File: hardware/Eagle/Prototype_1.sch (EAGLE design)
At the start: 11 parts, among them IC1 MEGA32-P, Q1 16MHz

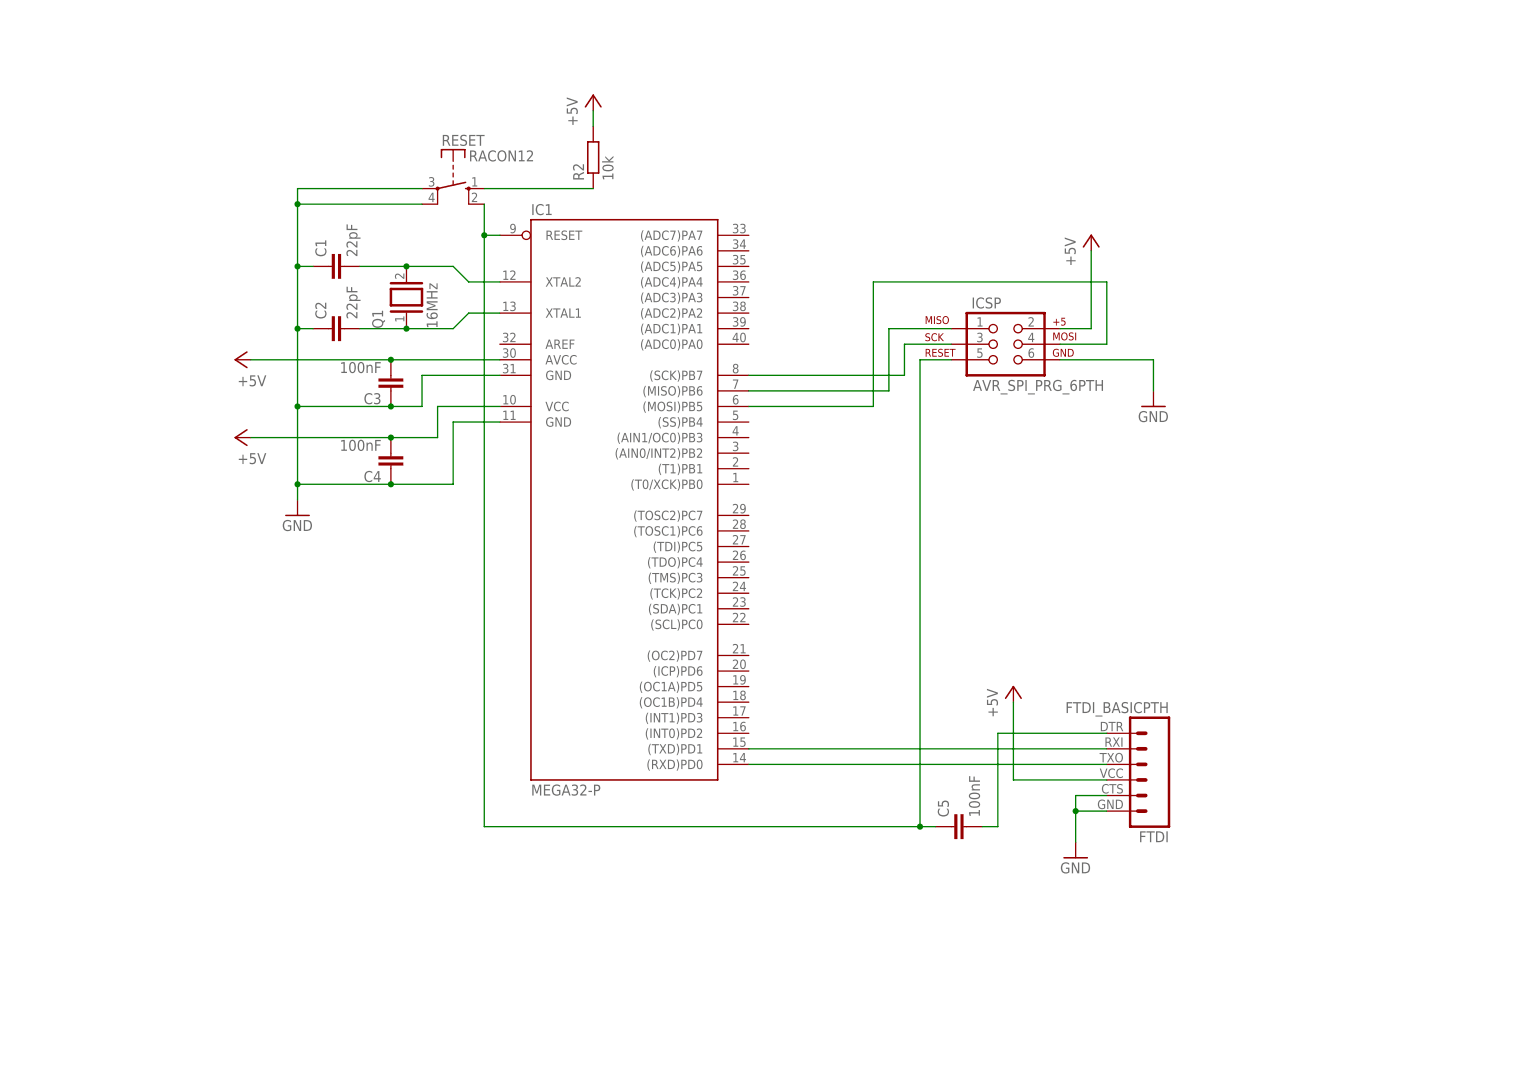
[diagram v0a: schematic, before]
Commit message: Readme and Eagle Circuit Files updated
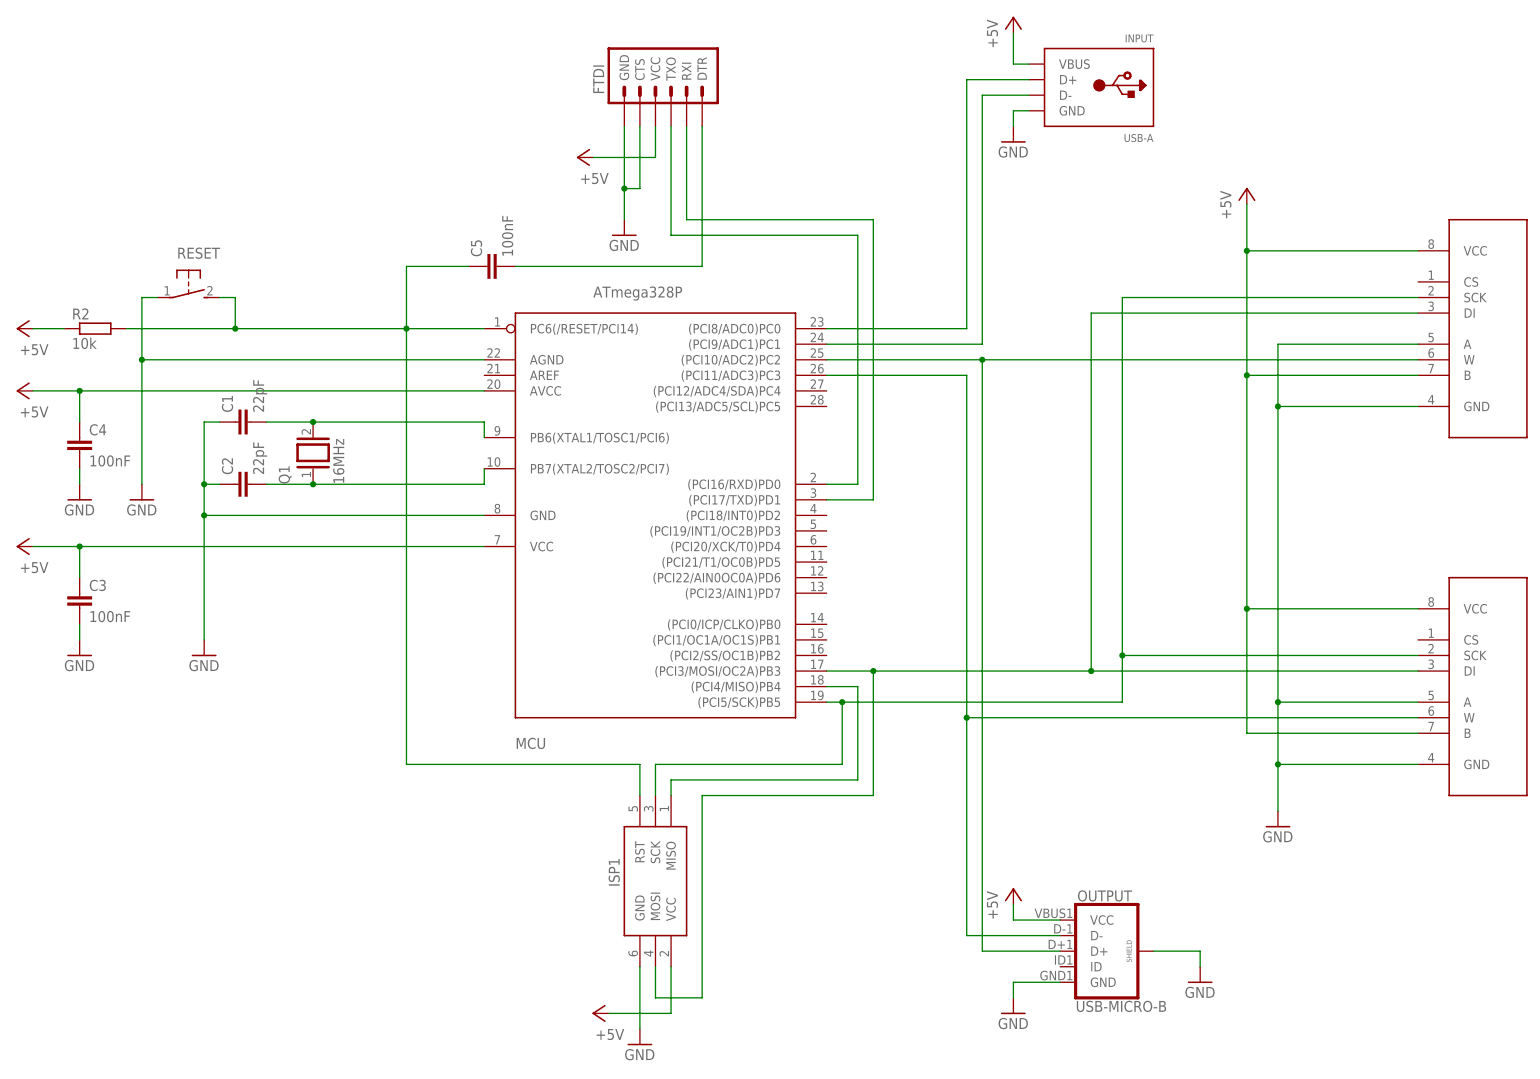
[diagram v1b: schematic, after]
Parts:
- removed IC1: MEGA32-P, atmel:MEGA32-P
- removed ICSP: AVR_SPI_PRG_6PTH, SparkFun-Connectors:AVR_SPI_PRG_6PTH
- added INPUT: USB-A, adafruit:USB-A
- added ISP1: AVRISP-6, adafruit:AVRISP-6
- added MCU: ATmega328P, adafruit:ATMEGA168-20P
- added OUTPUT: USB-MICRO-B, SparkFun-Connectors:USB_MICROB_PLUGCONN-11752
- added POTI, POTI1: MCP41XXXDIL, SparkFun-AnalogIC:MCP41XXXDIL
- FTDI: value FTDI_BASICPTH -> (none); device SparkFun-Connectors:FTDI_BASICPTH -> SparkFun-Connectors:ARDUINO_SERIAL_PROGRAMPTH
- RESET: value RACON12 -> (none); device switch-misc:RACON12 -> switch-omron:31-XX
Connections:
- removed net N$12: IC1.(MOSI)PB5, ICSP.4
- removed net N$6: FTDI.3, IC1.(RXD)PD0
- removed net N$7: R2.1, RESET.S
- removed net N$9: IC1.(MISO)PB6, ICSP.1
- new net MISO: ISP1.MISO, MCU.(PCI4/MISO)PB4
- new net MOSI: ISP1.MOSI, MCU.(PCI3/MOSI/OC2A)PB3, POTI.DI, POTI1.DI
- new net N$10: MCU.(PCI10/ADC2)PC2, OUTPUT.D+, POTI1.W
- new net N$11: MCU.(PCI11/ADC3)PC3, OUTPUT.D-, POTI.W
- new net N$14: INPUT.D+, MCU.(PCI8/ADC0)PC0
- new net N$15: INPUT.D-, MCU.(PCI9/ADC1)PC1
- new net SCK: ISP1.SCK, MCU.(PCI5/SCK)PB5, POTI.SCK, POTI1.SCK
- net +5V: now also C3.1, C4.1, FTDI.VCC, INPUT.VBUS, ISP1.VCC, MCU.AVCC, MCU.VCC, OUTPUT.VCC, POTI.B, POTI.VCC, POTI1.B, POTI1.VCC, R2.1; no longer C3.2, C4.2, FTDI.4, IC1.AVCC, IC1.VCC, ICSP.2, R2.2
- net GND: now also C3.2, C4.2, FTDI.CTS, FTDI.GND, INPUT.GND, ISP1.GND, MCU.AGND, MCU.GND, OUTPUT.GND, OUTPUT.SHIELD, POTI.A, POTI.GND, POTI1.A, POTI1.GND; no longer C3.1, C4.1, FTDI.5, FTDI.6, IC1.GND, IC1.GND@1, ICSP.6, RESET.P@1
- net N$1: now also C1.2, MCU.PB6(XTAL1/TOSC1/PCI6), Q1.2; no longer C2.2, IC1.XTAL1, Q1.1
- net N$2: now also C2.2, MCU.PB7(XTAL2/TOSC2/PCI7), Q1.1; no longer C1.2, IC1.XTAL2, Q1.2
- net N$3: now also FTDI.TXO, MCU.(PCI16/RXD)PD0; no longer C5.2, FTDI.1
- net N$4: now also ISP1.RST, MCU.PC6(/RESET/PCI14), R2.2, RESET.S; no longer IC1.RESET, ICSP.5, RESET.S@1
- net N$5: now also FTDI.RXI, MCU.(PCI17/TXD)PD1; no longer FTDI.2, IC1.(TXD)PD1
- net N$8: now also C5.2, FTDI.DTR; no longer IC1.(SCK)PB7, ICSP.3
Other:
- moved on the sheet: C1, C2, C3, C4, C5, FTDI, Q1, R2
